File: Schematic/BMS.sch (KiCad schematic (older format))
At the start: 0 parts

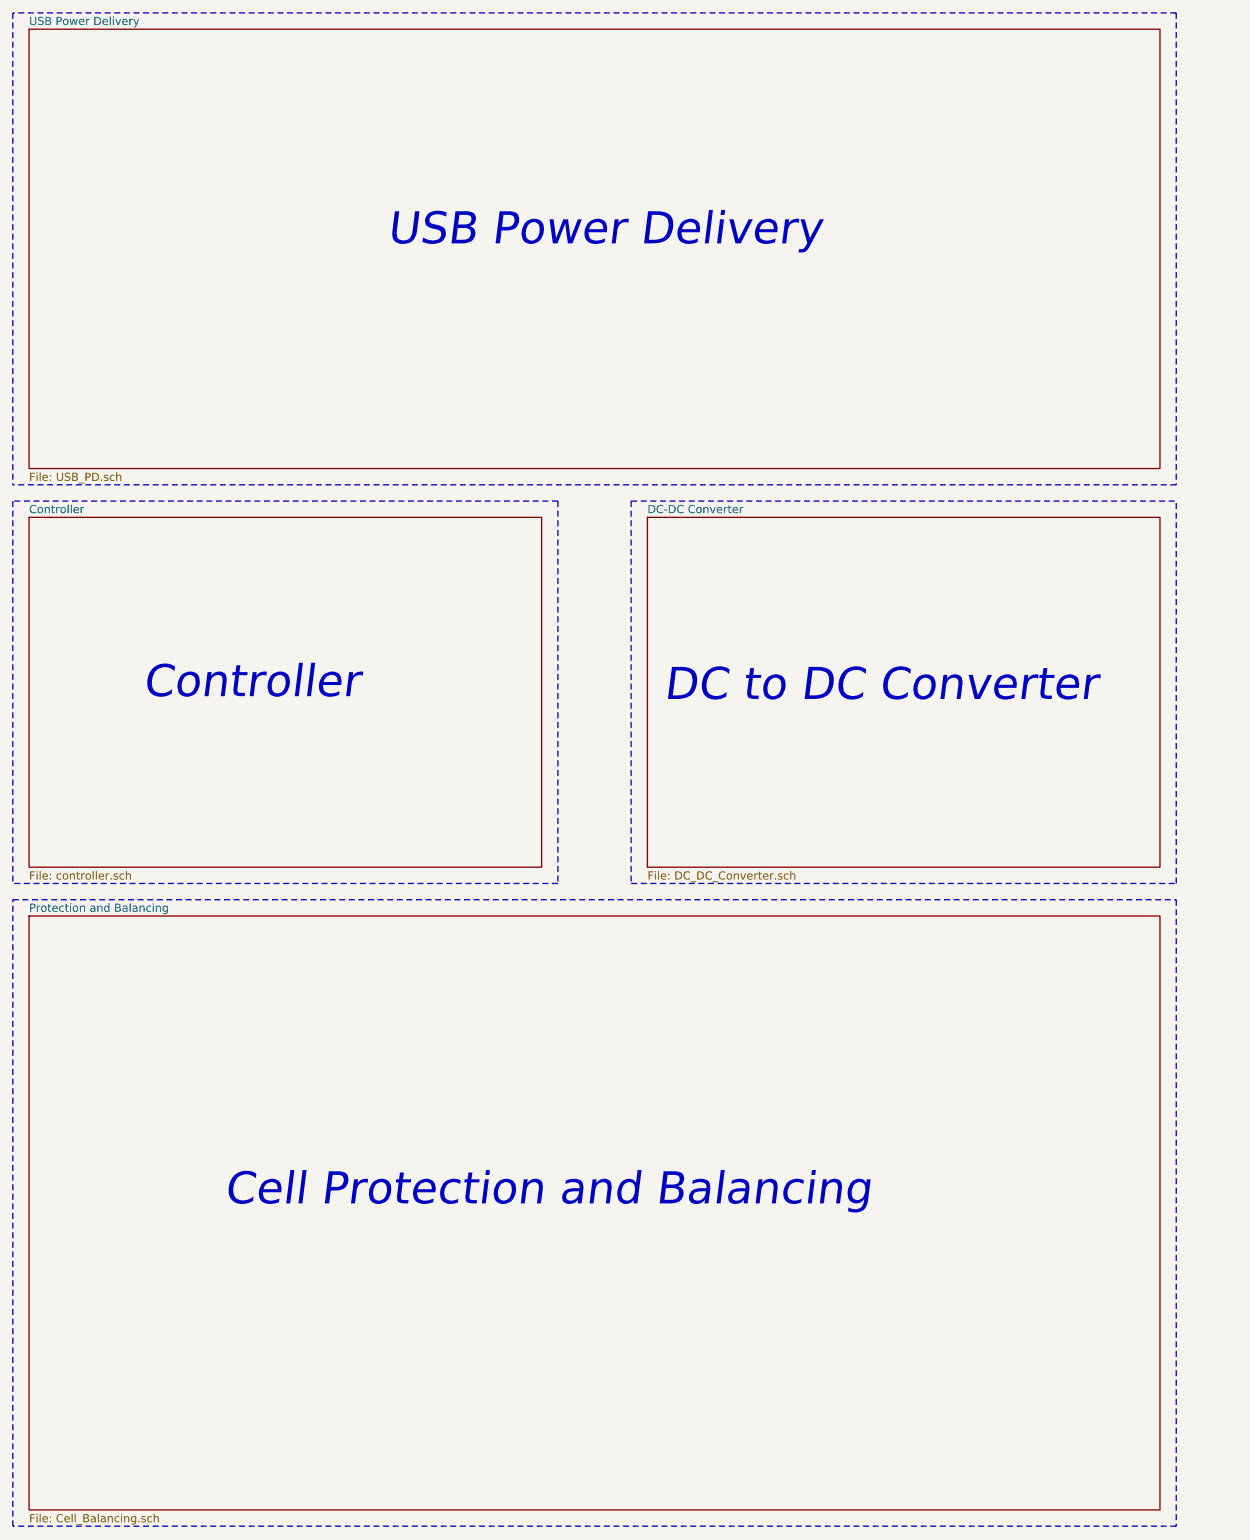
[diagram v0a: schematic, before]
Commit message: Add files via upload
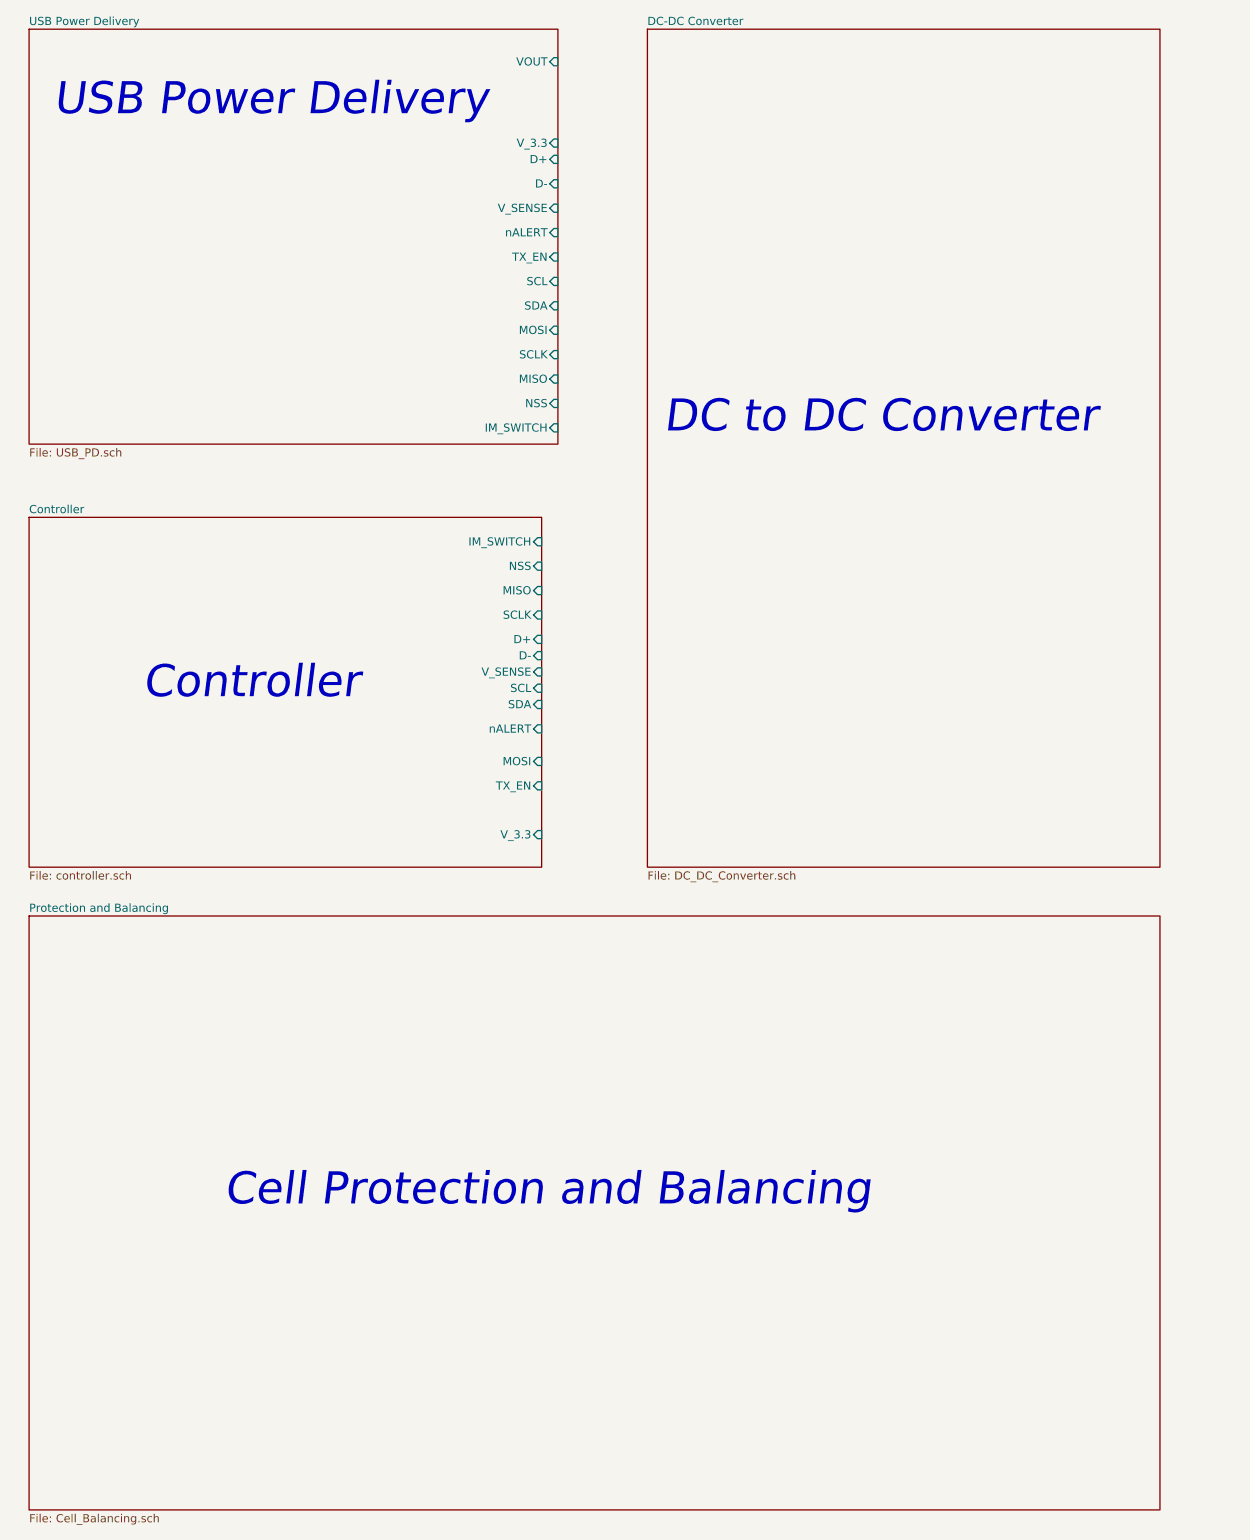
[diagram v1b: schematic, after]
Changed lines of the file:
@@
 Comment4 ""
 $EndDescr
-Wire Notes Line
-	550  550  550  3450
-Wire Notes Line
-	7700 550  550  550
-Wire Notes Line
-	7700 550  7700 3450
-Wire Notes Line
-	7700 3450 550  3450
 $Sheet
-S 650  650  6950 2700
+S 650  650  3250 2550
 U 5EFB5435
 F0 "USB Power Delivery" 50
 F1 "USB_PD.sch" 50
+F2 "IM_SWITCH" I R 3900 3100 50
+F3 "D+" I R 3900 1450 50
+F4 "D-" I R 3900 1600 50
+F5 "V_SENSE" I R 3900 1750 50
+F6 "VOUT" I R 3900 850 50
+F7 "SCL" I R 3900 2200 50
+F8 "SDA" I R 3900 2350 50
+F9 "nALERT" I R 3900 1900 50
+F10 "MOSI" I R 3900 2500 50
+F11 "TX_EN" I R 3900 2050 50
+F12 "SCLK" I R 3900 2650 50
+F13 "NSS" I R 3900 2950 50
+F14 "MISO" I R 3900 2800 50
+F15 "V_3.3" I R 3900 1350 50
 $EndSheet
-Text Notes 2850 2000 0    197  Italic 0
+Text Notes 800  1200 0    197  Italic 0
 USB Power Delivery
-Wire Notes Line
-	550  3550 550  5900
-Wire Notes Line
-	7700 5900 7700 3550
-Wire Notes Line
-	4350 3550 7700 3550
-Wire Notes Line
-	3900 3550 550  3550
-Wire Notes Line
-	4350 5900 7700 5900
-Wire Notes Line
-	4350 3550 4350 5900
-Wire Notes Line
-	3900 5900 550  5900
-Wire Notes Line
-	3900 3550 3900 5900
 $Sheet
-S 4450 3650 3150 2150
+S 4450 650  3150 5150
 U 5EFB8CA8
 F0 "DC-DC Converter" 50
 F1 "DC_DC_Converter.sch" 50
 $EndSheet
-Text Notes 4550 4800 0    197  Italic 0
+Text Notes 4550 3150 0    197  Italic 0
 DC to DC Converter\n
 Text Notes 1350 5100 0    197  Italic 0
@@
 F0 "Controller" 50
 F1 "controller.sch" 50
+F2 "IM_SWITCH" I R 3800 3800 50
+F3 "D+" I R 3800 4400 50
+F4 "D-" I R 3800 4500 50
+F5 "V_SENSE" I R 3800 4600 50
+F6 "SCL" I R 3800 4700 50
+F7 "SDA" I R 3800 4800 50
+F8 "nALERT" I R 3800 4950 50
+F9 "MOSI" I R 3800 5150 50
+F10 "TX_EN" I R 3800 5300 50
+F11 "SCLK" I R 3800 4250 50
+F12 "NSS" I R 3800 3950 50
+F13 "MISO" I R 3800 4100 50
+F14 "V_3.3" I R 3800 5600 50
 $EndSheet
-Wire Notes Line
-	550  6000 7700 6000
-Wire Notes Line
-	7700 6000 7700 9850
-Wire Notes Line
-	7700 9850 550  9850
-Wire Notes Line
-	550  9850 550  6000
+Text Notes 1850 7900 0    197  Italic 0
+Cell Protection and Balancing
 $Sheet
 S 650  6100 6950 3650
@@
 F1 "Cell_Balancing.sch" 50
 $EndSheet
-Text Notes 1850 7900 0    197  Italic 0
-Cell Protection and Balancing
 $EndSCHEMATC
